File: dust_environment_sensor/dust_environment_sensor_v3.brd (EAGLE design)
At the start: 63.5 x 30.5 mm, 38 parts, among them IC2 ATMEGA644A, J1 3.6V Lithium C cell, J3 XBEE_1-10SMT, J4 XBEE_11-20SMT, U1 TSL2560T, U2 LIS3DH, U4 HTU21D, U5 AMN41121, U7 MCP1700-3.3V, X2 32.768KHz

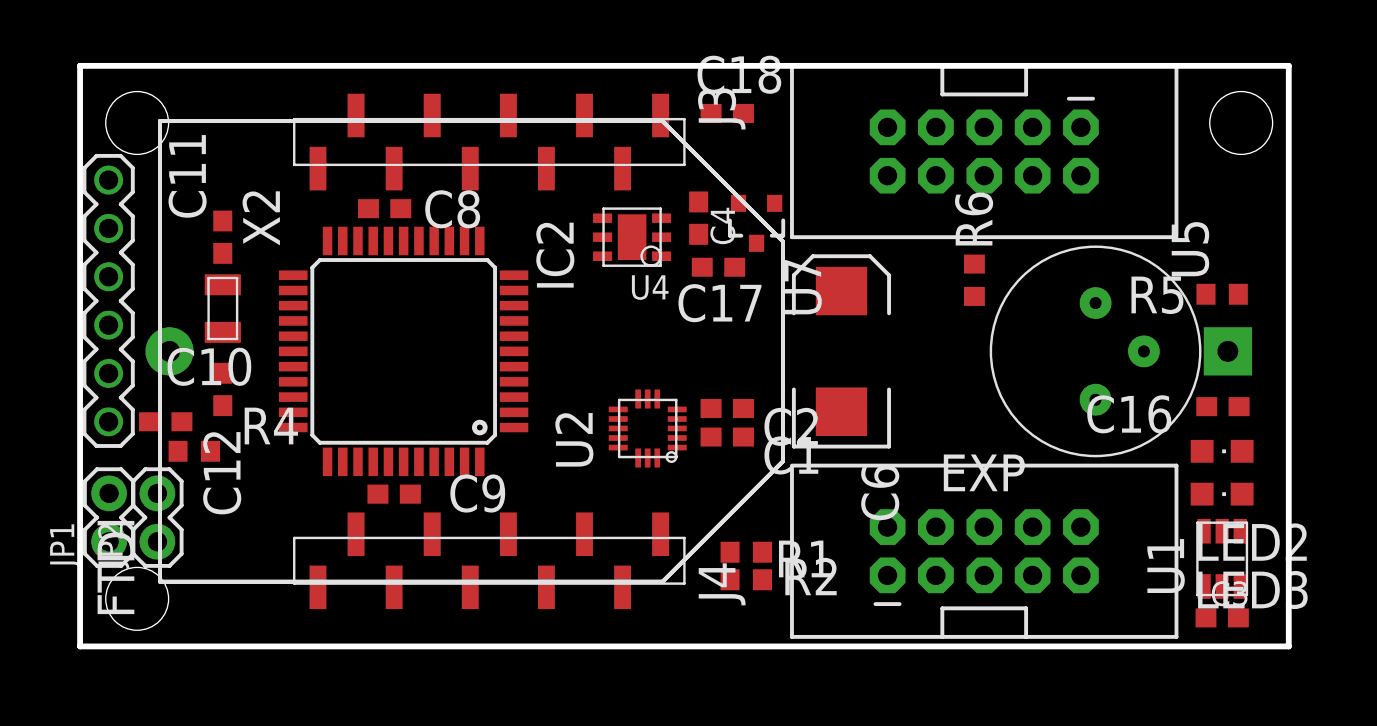
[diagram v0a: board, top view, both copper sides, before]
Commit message: boards submitted to fab
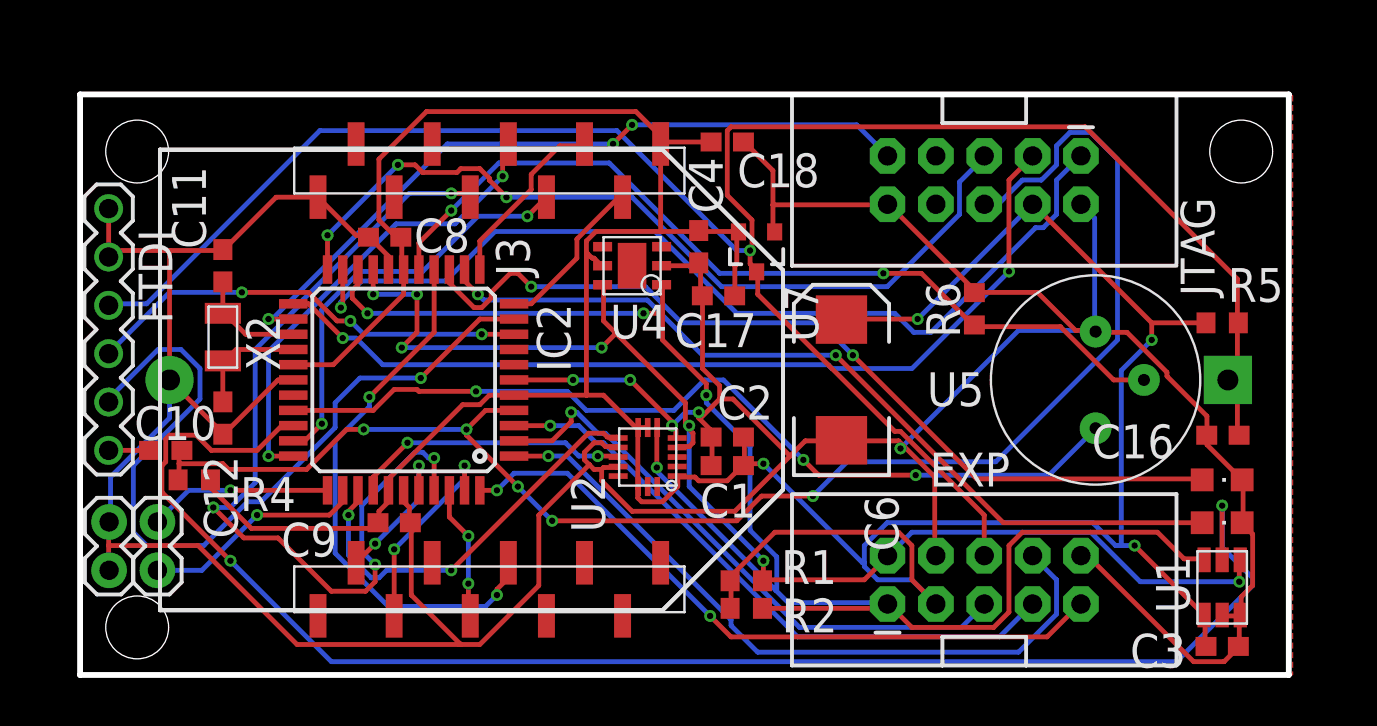
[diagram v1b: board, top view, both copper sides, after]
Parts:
- LED2: value (none) -> BLUE
- LED3: value (none) -> AMBER
- moved C1 1.50 mm to (34.0, 11.0)
- moved C10 1.50 mm to (4.50, 11.8)
- moved C11 1.50 mm to (7.50, 21.5)
- moved C12 1.50 mm to (7.50, 13.5)
- moved C16 1.50 mm to (60.0, 12.6)
- moved C17 1.50 mm to (33.5, 19.9)
- moved C18 1.50 mm to (34.0, 28.0)
- moved C2 1.50 mm to (34.0, 12.5)
- moved C3 1.50 mm to (60.0, 1.50)
- moved C4 1.50 mm to (32.5, 22.5)
- moved C6 1.50 mm to (40.0, 15.5)
- moved C8 1.50 mm to (16.0, 23.0)
- moved C9 1.50 mm to (16.5, 8.00)
- moved EXP 1.50 mm to (47.5, 5.00)
- moved IC2 1.50 mm to (17.0, 15.5)
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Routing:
- net GND: track 0.00 -> 230.2 mm, vias 0 -> 5
- net VCC: track 0.00 -> 190.5 mm, vias 0 -> 4
- net VBATT: track 0.00 -> 108.2 mm, vias 0 -> 1
- net I2C_SDA: track 0.00 -> 82.7 mm, vias 0 -> 4
- net LIGHT_INT: track 0.00 -> 80.9 mm, vias 0 -> 2
- net RST: track 0.00 -> 80.2 mm, vias 0 -> 5
- net I2C_SCL: track 0.00 -> 67.9 mm, vias 0 -> 7
- net TCK: track 0.00 -> 49.8 mm, vias 0 -> 1
- net TDO: track 0.00 -> 47.7 mm, vias 0 -> 2
- net PIR_VCC: track 0.00 -> 46.8 mm, vias 0 -> 3
- net MOTE_CONNECT: track 0.00 -> 46.2 mm, vias 0 -> 4
- net LED1: track 0.00 -> 46.2 mm, vias 0 -> 2
- net PIR_OUT: track 0.00 -> 46.0 mm, vias 0 -> 2
- net LED2: track 0.00 -> 44.6 mm, vias 0 -> 2
- net TMS: track 0.00 -> 44.6 mm, vias 0 -> 3
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- added copper zone on layer 1, net GND
- added copper zone on layer 16, net GND
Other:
- board text added: "JTAG"

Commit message: Updated board design and shipping
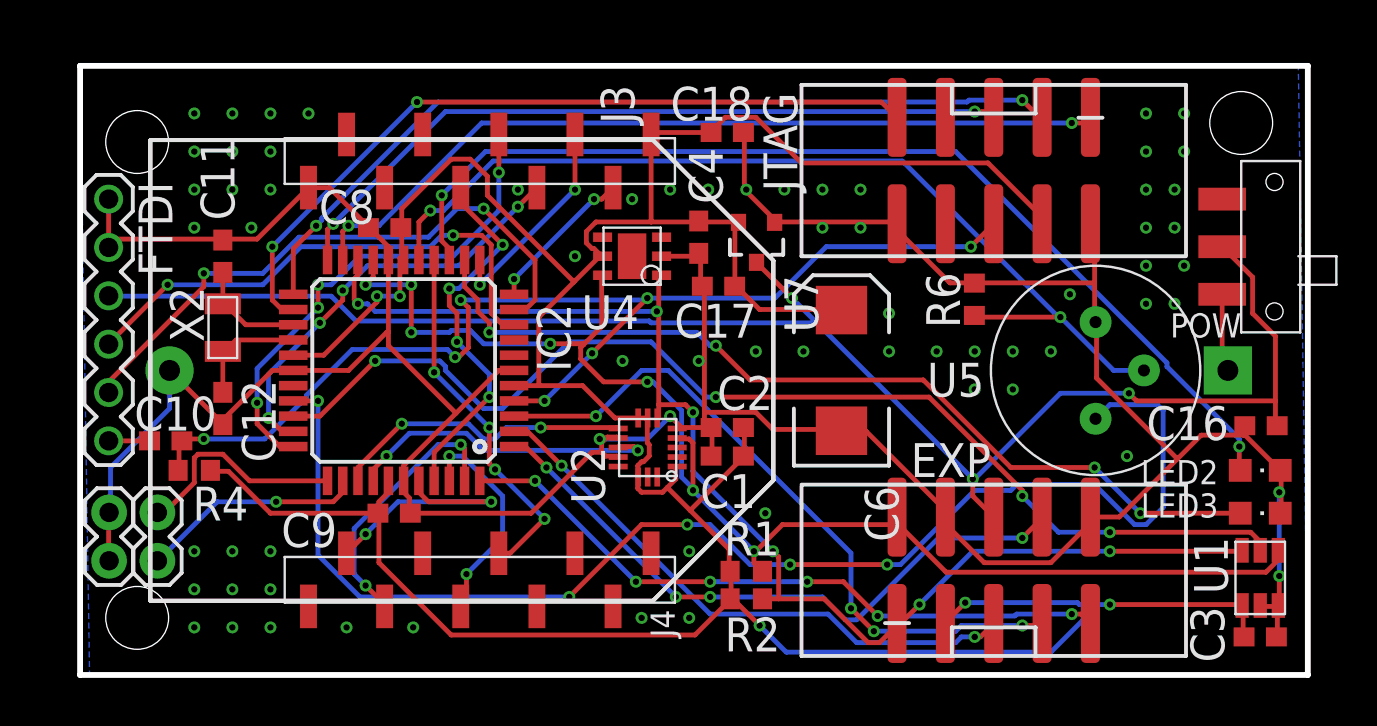
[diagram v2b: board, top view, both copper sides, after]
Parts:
- removed R5: 0R DNP, resistor:R0603
- added POW: POWER, Cool_Electricity:JS102011SAQN
- EXP: value M05X2SHD -> M05X2SHD_SMD; device SparkFun-Connectors:2X5-SHROUDED -> SparkFun-Connectors:2X5-SHROUDED_SMD
- JP9: device SparkFun-Connectors:2X5-SHROUDED -> SparkFun-Connectors:2X5-SHROUDED_SMD
- moved C16 2.06 mm to (62.0, 13.1)
- moved C3 2.06 mm to (62.0, 2.00)
- moved LED2 2.06 mm to (62.0, 10.8)
- moved LED3 2.06 mm to (62.0, 8.50)
- moved U1 2.06 mm to (62.0, 5.10)
- moved STANDOFF1 1.50 mm to (61.0, 29.0)
- moved EXP 0.71 mm to (48.0, 5.50)
- moved J3 0.71 mm to (21.0, 16.0)
- moved J4 0.71 mm to (21.0, 16.0)
- moved JP9 0.71 mm to (48.0, 26.5)
- moved C1 0.50 mm to (34.0, 11.5)
- moved C10 0.50 mm to (4.50, 12.3)
- moved C11 0.50 mm to (7.50, 22.0)
- moved C12 0.50 mm to (7.50, 14.0)
- moved C17 0.50 mm to (33.5, 20.4)
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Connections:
- new net N$1: J1.POS, POW.1
- net VBATT: now also POW.C; no longer J1.POS, R5.2
- net VCC: no longer R5.1
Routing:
- net GND: track 230.2 -> 189.7 mm, vias 5 -> 68
- net MOTE_CONNECT: track 46.2 -> 19.8 mm
- net VBATT: track 108.2 -> 84.9 mm, vias 1 -> 3
- net PIR_VCC: track 46.8 -> 69.2 mm, vias 3 -> 5
- net LIGHT_INT: track 80.9 -> 59.6 mm, vias 2 -> 4
- net RST: track 80.2 -> 60.8 mm, vias 5 -> 7
- net I2C_SDA: track 82.7 -> 68.1 mm, vias 4 -> 6
- net ATMEGA_TO_FTDI: track 42.5 -> 31.7 mm, vias 1 -> 2
- net MOTE_RX_RTSN: track 28.9 -> 19.2 mm, vias 2 -> 4
- net LED1: track 46.2 -> 54.5 mm
- net VCC: track 190.5 -> 183.4 mm, vias 4 -> 5
- net TCK: track 49.8 -> 43.3 mm, vias 1 -> 2
- net ACCEL_INT2: track 21.5 -> 15.9 mm
- net MOTE_TX_CTSN: track 7.77 -> 13.3 mm
- net TMS: track 44.6 -> 39.3 mm, vias 3 -> 2
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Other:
- board size 63.5 x 30.5 mm -> 64.5 x 32 mm
- board text added: "ESENSE v3.1 Kevin Weekly"
- board text removed: "Environmental Sensor PCB Kevin Weekly"
